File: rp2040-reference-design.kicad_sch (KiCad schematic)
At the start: 31 parts, among them J1 Conn_02x05_Odd_Even, SW1 SW_Push, SW2 SW_Push, U1 RP2040, U2 W25Q128JVS, Y1 12mhz ABM8-272-T

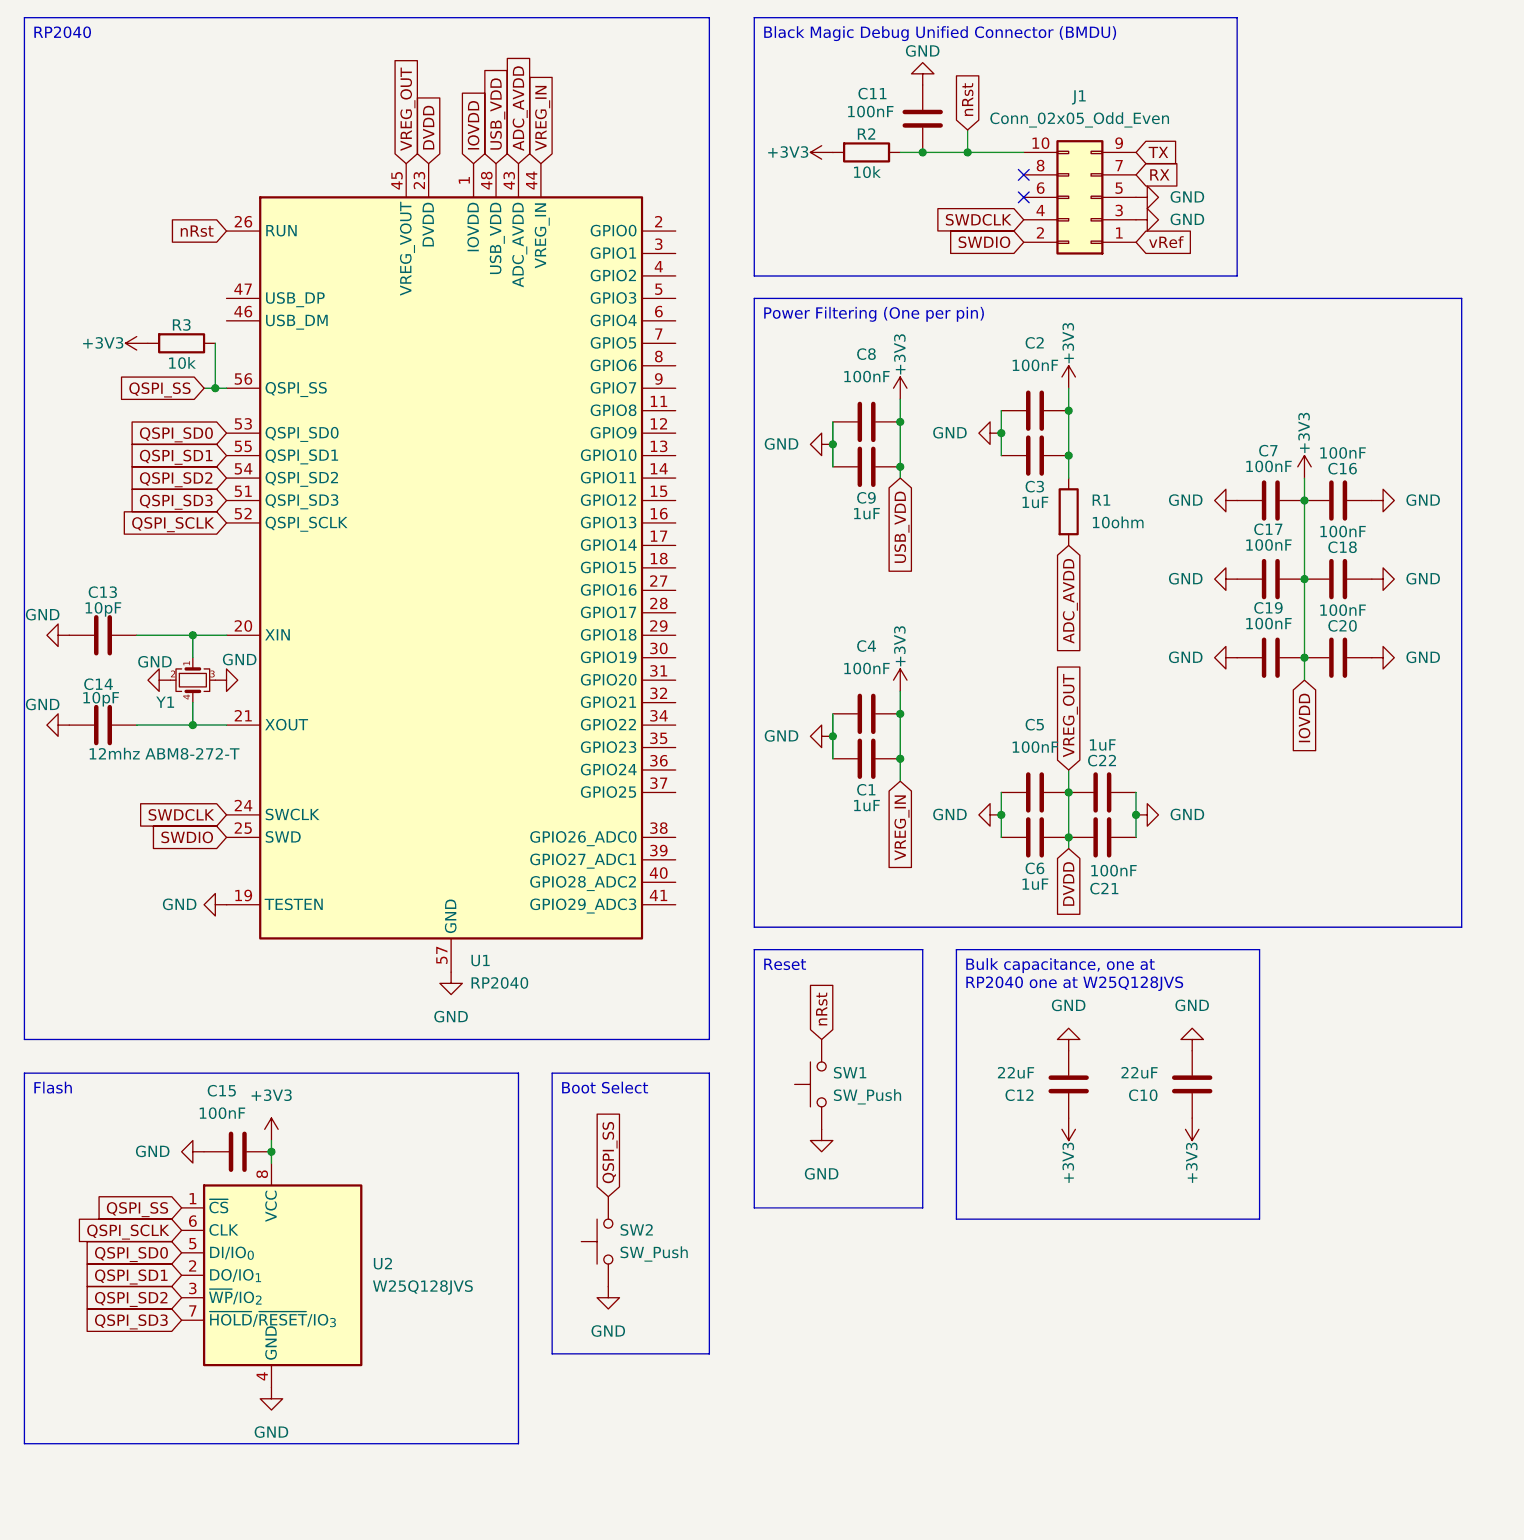
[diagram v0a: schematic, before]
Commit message: feat: led
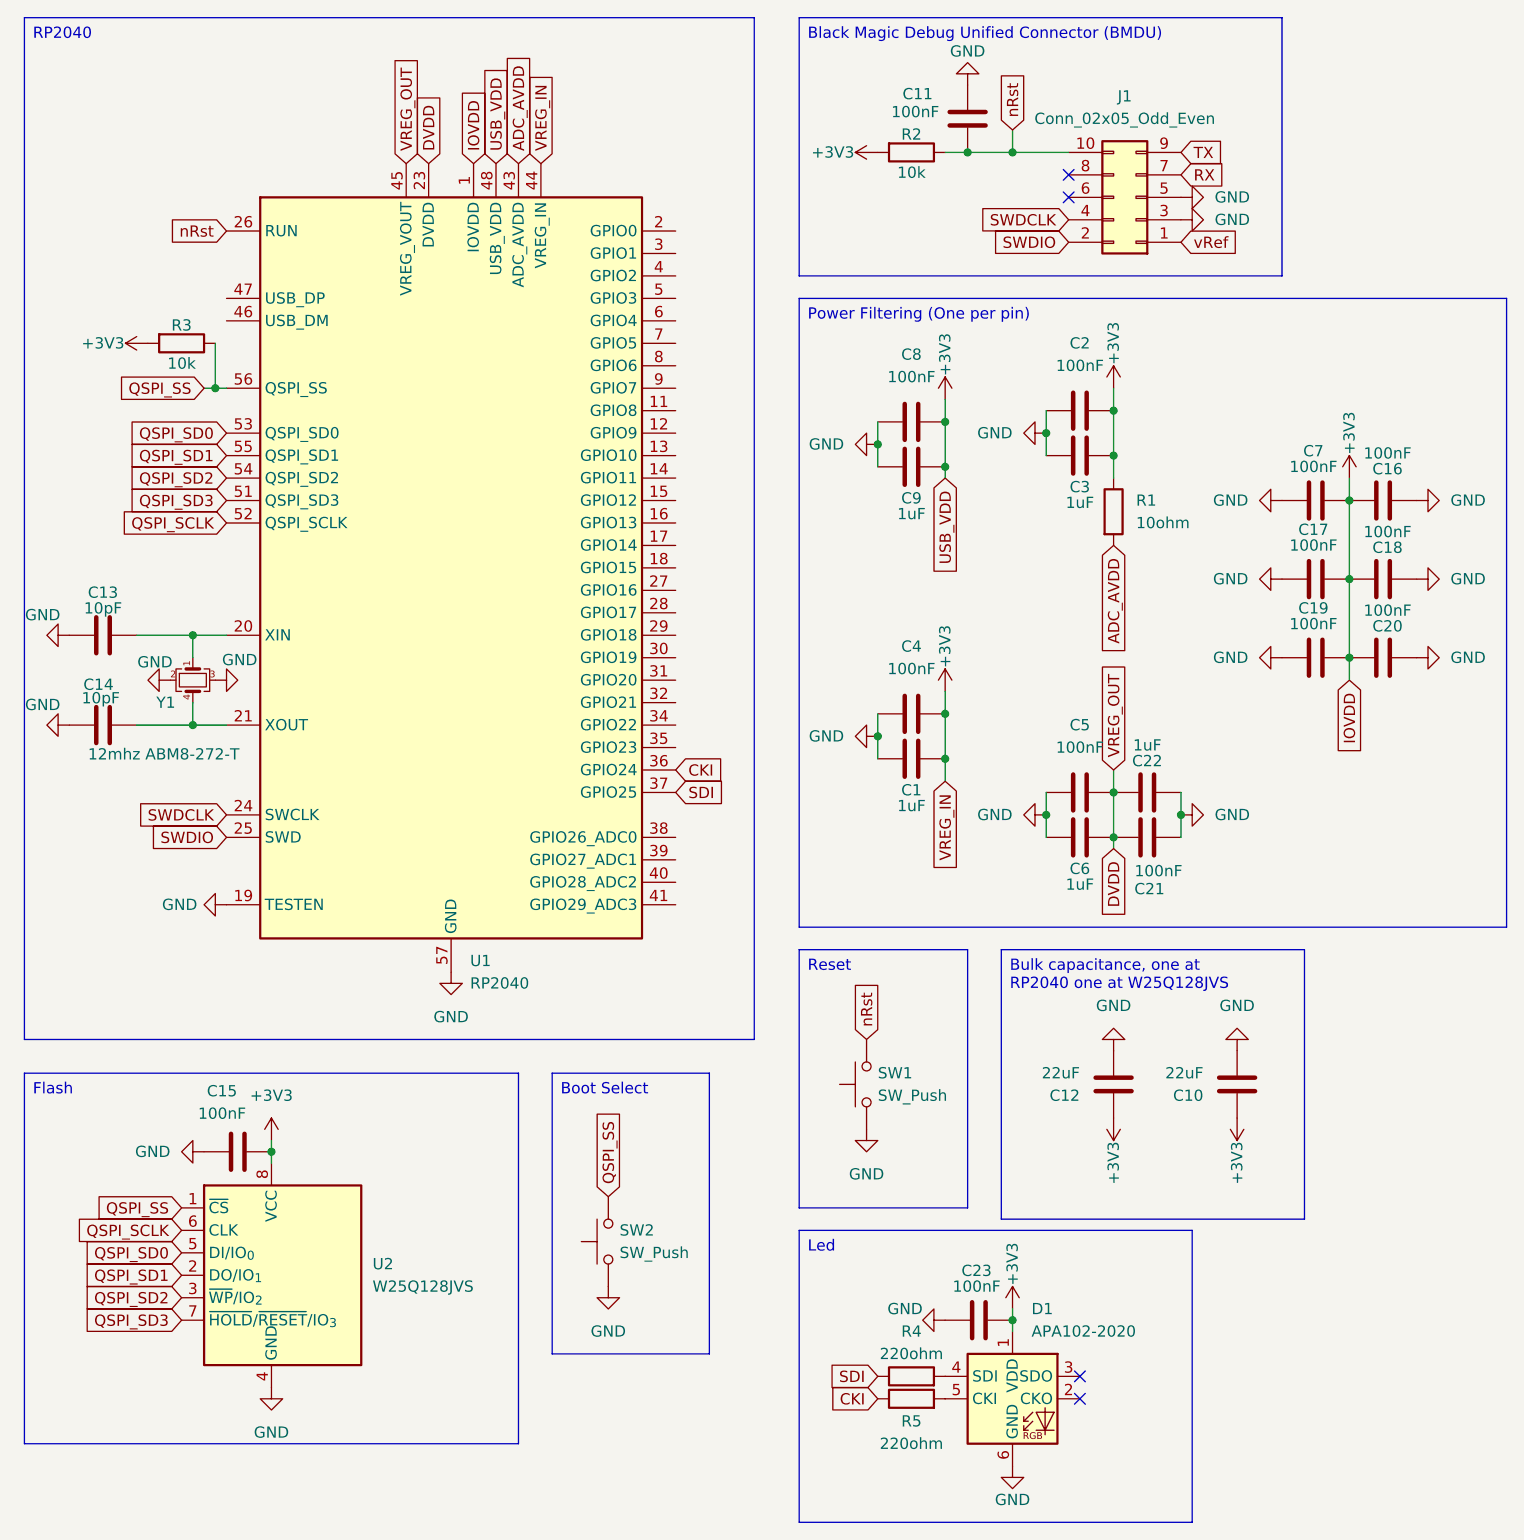
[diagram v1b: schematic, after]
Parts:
- added C23: 100nF, Capacitor_SMD:C_0402_1005Metric, symbol Device:C
- added D1: APA102-2020, LED_SMD:LED-APA102-2020, symbol LED:APA102-2020
- added R4, R5: 220ohm, Resistor_SMD:R_0402_1005Metric, symbol Device:R
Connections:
- net +3V3: now also C23.2, D1.1 (VDD)
- net GND: now also C23.1, D1.6 (GND)
- net CKI: now reaches U1.36 (GPIO24)
- net CKI: now also R5.1
- net SDI: now reaches U1.37 (GPIO25)
- net SDI: now also R4.1
- new net: D1.4 (SDI), R4.2
- new net: D1.5 (CKI), R5.2
- no-connect marks 2 -> 4
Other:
- moved on the sheet: C1, C10, C11, C12, C16, C17, C18, C19, C2, C20, C21, C22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
